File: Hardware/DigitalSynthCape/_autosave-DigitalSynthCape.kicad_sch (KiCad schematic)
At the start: 20 parts, among them J1 Conn_01x01_Male, P9 BeagleBone_Black_Header

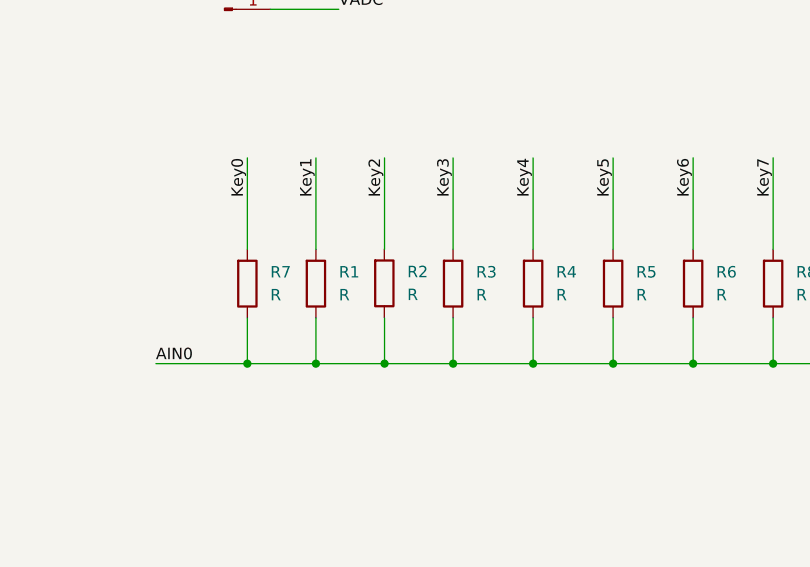
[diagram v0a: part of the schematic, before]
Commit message: Updates to PCB
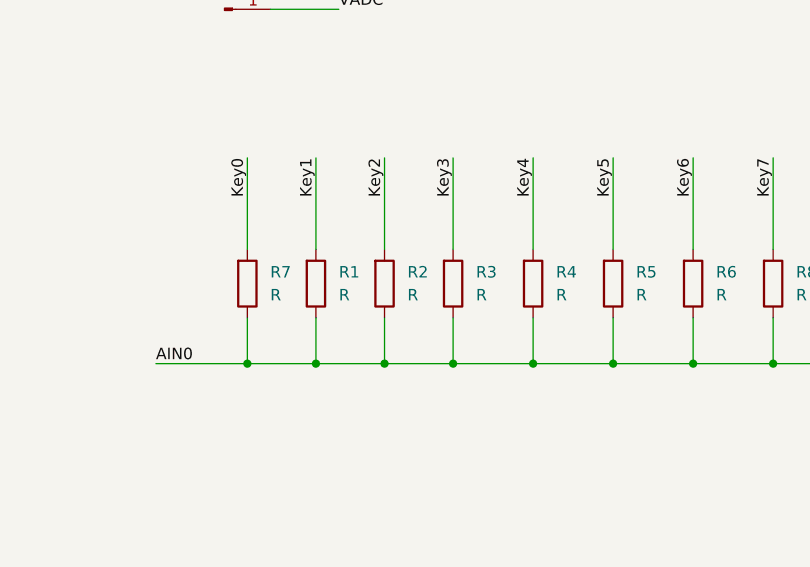
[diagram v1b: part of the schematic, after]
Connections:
- net AIN0: now also R2.2
- net Key2: now also R2.1
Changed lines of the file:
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@@
+    )
+  )
+  (symbol (lib_id "Resistors:R") (at 135.89 133.35 0) (unit 1)
+    (in_bom yes) (on_board yes) (dnp no) (fields_autoplaced)
+    (property "Reference" "R2" (at 138.43 132.08 0)
+      (effects (font (size 1.27 1.27)) (justify left))
+    )
+    (property "Value" "R" (at 138.43 134.62 0)
+      (effects (font (size 1.27 1.27)) (justify left))
+    )
+    (property "Footprint" "Resistor_SMD:R_1206_3216Metric" (at 135.89 152.4 0)
+      (effects (font (size 1.27 1.27)) hide)
+    )
+    (property "Datasheet" "" (at 134.62 147.32 0)
+      (effects (font (size 1.27 1.27)) hide)
+    )
+    (pin "1")
+    (pin "2")
+    (instances
+      (project "DigitalSynthCape"
+        (path "/e63e39d7-6ac0-4ffd-8aa3-1841a4541b55"
+          (reference "R2") (unit 1)
+        )
+      )
     )
   )
@@
         )
       )
-    )
-  )
-  (symbol (lib_id "Resistors:R") (at 135.8681 133.3196 0) (unit 1)
-    (in_bom yes) (on_board yes) (dnp no) (fields_autoplaced)
-    (property "Reference" "R2" (at 138.4081 132.0496 0)
-      (effects (font (size 1.27 1.27)) (justify left))
-    )
-    (property "Value" "R" (at 138.4081 134.5896 0)
-      (effects (font (size 1.27 1.27)) (justify left))
-    )
-    (property "Footprint" "Resistor_SMD:R_1206_3216Metric" (at 135.8681 152.3696 0)
-      (effects (font (size 1.27 1.27)) hide)
-    )
-    (property "Datasheet" "" (at 134.5981 147.2896 0)
-      (effects (font (size 1.27 1.27)) hide)
-    )
-    (pin "1")
-    (pin "2")
-    (instances
-      (project "DigitalSynthCape"
-        (path "/e63e39d7-6ac0-4ffd-8aa3-1841a4541b55"
-          (reference "R2") (unit 1)
-        )
-      )
